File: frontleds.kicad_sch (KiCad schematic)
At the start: 2 parts

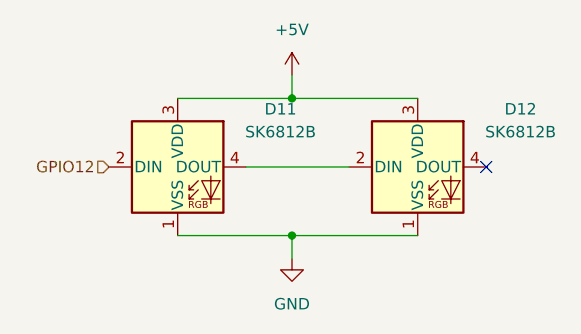
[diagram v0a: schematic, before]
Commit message: finished adding front leds
probably works idk
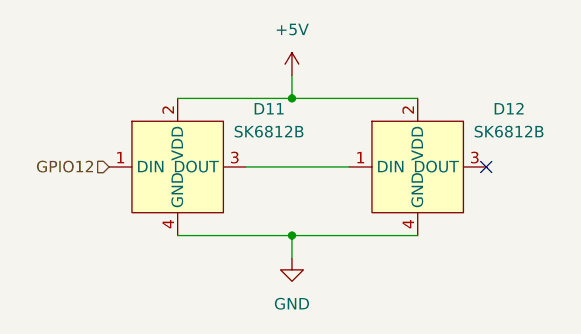
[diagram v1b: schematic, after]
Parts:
- D11, D12: footprint LED_SMD:LED_SK6812_PLCC4_5.0x5.0mm_P3.2mm -> LED_SMD:LED_SK6812B_SIDE_4.0mmx1.5mm
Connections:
- net +5V: now also D11.2 (VDD), D12.2 (VDD); no longer D11.3 (VDD), D12.3 (VDD)
- net GND: now also D11.4 (GND), D12.4 (GND); no longer D11.1 (VSS), D12.1 (VSS)
- net GPIO12: now also D11.1 (DIN); no longer D11.2 (DIN)
- new net: D11.3 (DOUT), D12.1 (DIN)
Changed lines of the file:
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@@
+	)
+	(symbol
+		(lib_id "LED:SK6812B")
+		(at 55.88 29.21 0)
+		(unit 1)
+		(exclude_from_sim no)
+		(in_bom yes)
+		(on_board yes)
+		(dnp no)
+		(fields_autoplaced yes)
+		(property "Reference" "D12"
+			(at 66.04 22.7898 0)
+			(effects
+				(font
+					(size 1.27 1.27)
+				)
+			)
+		)
+		(property "Value" "SK6812B"
+			(at 66.04 25.3298 0)
+			(effects
+				(font
+					(size 1.27 1.27)
+				)
+			)
+		)
+		(property "Footprint" "LED_SMD:LED_SK6812B_SIDE_4.0mmx1.5mm"
+			(at 55.88 29.21 0)
+			(effects
+				(font
+					(size 1.27 1.27)
+				)
+				(hide yes)
+			)
+		)
+		(property "Datasheet" "https://core-electronics.com.au/attachments/localcontent/4691_SK68XX_SIDE_REV_55747b5a68c.pdf"
+			(at 55.88 10.16 0)
+			(effects
+				(font
+					(size 1.27 1.27)
+				)
+				(hide yes)
+			)
+		)
+		(property "Description" "RGB LED with integrated controller"
+			(at 55.88 7.62 0)
+			(effects
+				(font
+					(size 1.27 1.27)
+				)
+				(hide yes)
+			)
+		)
+		(pin "3"
+		)
+		(pin "1"
+		)
+		(pin "4"
+		)
+		(pin "2"
+		)
+		(instances
+			(project "robot_pcb"
+				(path "/2f56b371-1597-47e1-a48d-b7f69d342f77/f9fd353d-136c-4b1d-af31-404dc5242855"
+					(reference "D12")
+					(unit 1)
+				)
+			)
+		)
 	)
 	(symbol
@@
 	)
 	(symbol
+		(lib_id "power:GND")
+		(at 41.91 39.37 0)
+		(unit 1)
+		(exclude_from_sim no)
+		(in_bom yes)
+		(on_board yes)
+		(dnp no)
+		(fields_autoplaced yes)
+		(property "Reference" "#PWR0121"
+			(at 41.91 45.72 0)
+			(effects
+				(font
+					(size 1.27 1.27)
+				)
+				(hide yes)
+			)
+		)
+		(property "Value" "GND"
+			(at 41.91 44.45 0)
+			(effects
+				(font
+					(size 1.27 1.27)
+				)
+			)
+		)
+		(property "Footprint" ""
+			(at 41.91 39.37 0)
+			(effects
+				(font
+					(size 1.27 1.27)
+				)
+				(hide yes)
+			)
+		)
+		(property "Datasheet" ""
+			(at 41.91 39.37 0)
+			(effects
+				(font
+					(size 1.27 1.27)
+				)
+				(hide yes)
+			)
+		)
+		(property "Description" "Power symbol creates a global label with name \"GND\" , ground"
+			(at 41.91 39.37 0)
+			(effects
+				(font
+					(size 1.27 1.27)
+				)
+				(hide yes)
+			)
+		)
+		(pin "1"
+		)
+		(instances
+			(project ""
+				(path "/2f56b371-1597-47e1-a48d-b7f69d342f77/f9fd353d-136c-4b1d-af31-404dc5242855"
+					(reference "#PWR0121")
+					(unit 1)
+				)
+			)
+		)
+	)
+	(symbol
 		(lib_id "LED:SK6812B")
 		(at 29.21 29.21 0)
@@
 		(fields_autoplaced yes)
 		(property "Reference" "D11"
-			(at 40.64 22.7898 0)
+			(at 39.37 22.7898 0)
 			(effects
 				(font
@@
 		)
 		(property "Value" "SK6812B"
-			(at 40.64 25.3298 0)
-			(effects
-				(font
-					(size 1.27 1.27)
-				)
-			)
-		)
-		(property "Footprint" "LED_SMD:LED_SK6812_PLCC4_5.0x5.0mm_P3.2mm"
-			(at 30.48 36.83 0)
-			(effects
-				(font
-					(size 1.27 1.27)
-				)
-				(justify left top)
+			(at 39.37 25.3298 0)
+			(effects
+				(font
+					(size 1.27 1.27)
+				)
+			)
+		)
+		(property "Footprint" "LED_SMD:LED_SK6812B_SIDE_4.0mmx1.5mm"
+			(at 29.21 29.21 0)
+			(effects
+				(font
+					(size 1.27 1.27)
+				)
 				(hide yes)
 			)
 		)
 		(property "Datasheet" "https://core-electronics.com.au/attachments/localcontent/4691_SK68XX_SIDE_REV_55747b5a68c.pdf"
-			(at 31.75 38.735 0)
-			(effects
-				(font
-					(size 1.27 1.27)
-				)
-				(justify left top)
-				(hide yes)
-			)
-		)
-		(property "Description" "Side-light RGB LED with integrated controller"
-			(at 29.21 29.21 0)
-			(effects
-				(font
-					(size 1.27 1.27)
-				)
-				(hide yes)
-			)
+			(at 29.21 10.16 0)
+			(effects
+				(font
+					(size 1.27 1.27)
+				)
+				(hide yes)
+			)
+		)
+		(property "Description" "RGB LED with integrated controller"
+			(at 29.21 7.62 0)
+			(effects
+				(font
+					(size 1.27 1.27)
+				)
+				(hide yes)
+			)
+		)
+		(pin "3"
+		)
+		(pin "1"
+		)
+		(pin "4"
 		)
 		(pin "2"
 		)
-		(pin "1"
-		)
-		(pin "4"
-		)
-		(pin "3"
-		)
 		(instances
 			(project ""
@@
 					(unit 1)
 				)
-			)
-		)
-	)
-	(symbol
-		(lib_id "power:GND")
-		(at 41.91 39.37 0)
-		(unit 1)
-		(exclude_from_sim no)
-		(in_bom yes)
-		(on_board yes)
-		(dnp no)
-		(fields_autoplaced yes)
-		(property "Reference" "#PWR0121"
-			(at 41.91 45.72 0)
-			(effects
-				(font
-					(size 1.27 1.27)
-				)
-				(hide yes)
-			)
-		)
-		(property "Value" "GND"
-			(at 41.91 44.45 0)
-			(effects
-				(font
-					(size 1.27 1.27)
-				)
-			)
-		)
-		(property "Footprint" ""
-			(at 41.91 39.37 0)
-			(effects
-				(font
-					(size 1.27 1.27)
-				)
-				(hide yes)
-			)
-		)
-		(property "Datasheet" ""
-			(at 41.91 39.37 0)
-			(effects
-				(font
-					(size 1.27 1.27)
-				)
-				(hide yes)
-			)
-		)
-		(property "Description" "Power symbol creates a global label with name \"GND\" , ground"
-			(at 41.91 39.37 0)
-			(effects
-				(font
-					(size 1.27 1.27)
-				)
-				(hide yes)
-			)
-		)
-		(pin "1"
-		)
-		(instances
-			(project ""
-				(path "/2f56b371-1597-47e1-a48d-b7f69d342f77/f9fd353d-136c-4b1d-af31-404dc5242855"
-					(reference "#PWR0121")
-					(unit 1)
-				)
-			)
-		)
-	)
-	(symbol
-		(lib_id "LED:SK6812B")
-		(at 55.88 29.21 0)
-		(unit 1)
-		(exclude_from_sim no)
-		(in_bom yes)
-		(on_board yes)
-		(dnp no)
-		(fields_autoplaced yes)
-		(property "Reference" "D12"
-			(at 67.31 22.7898 0)
-			(effects
-				(font
-					(size 1.27 1.27)
-				)
-			)
-		)
-		(property "Value" "SK6812B"
-			(at 67.31 25.3298 0)
-			(effects
-				(font
-					(size 1.27 1.27)
-				)
-			)
-		)
-		(property "Footprint" "LED_SMD:LED_SK6812_PLCC4_5.0x5.0mm_P3.2mm"
-			(at 57.15 36.83 0)
-			(effects
-				(font
-					(size 1.27 1.27)
-				)
-				(justify left top)
-				(hide yes)
-			)
-		)
-		(property "Datasheet" "https://core-electronics.com.au/attachments/localcontent/4691_SK68XX_SIDE_REV_55747b5a68c.pdf"
-			(at 58.42 38.735 0)
-			(effects
-				(font
-					(size 1.27 1.27)
-				)
-				(justify left top)
-				(hide yes)
-			)
-		)
-		(property "Description" "Side-light RGB LED with integrated controller"
-			(at 55.88 29.21 0)
-			(effects
-				(font
-					(size 1.27 1.27)
-				)
-				(hide yes)
-			)
-		)
-		(pin "2"
-		)
-		(pin "1"
-		)
-		(pin "4"
-		)
-		(pin "3"
-		)
-		(instances
-			(project "robot_pcb"
-				(path "/2f56b371-1597-47e1-a48d-b7f69d342f77/f9fd353d-136c-4b1d-af31-404dc5242855"
-					(reference "D12")
-					(unit 1)
-				)

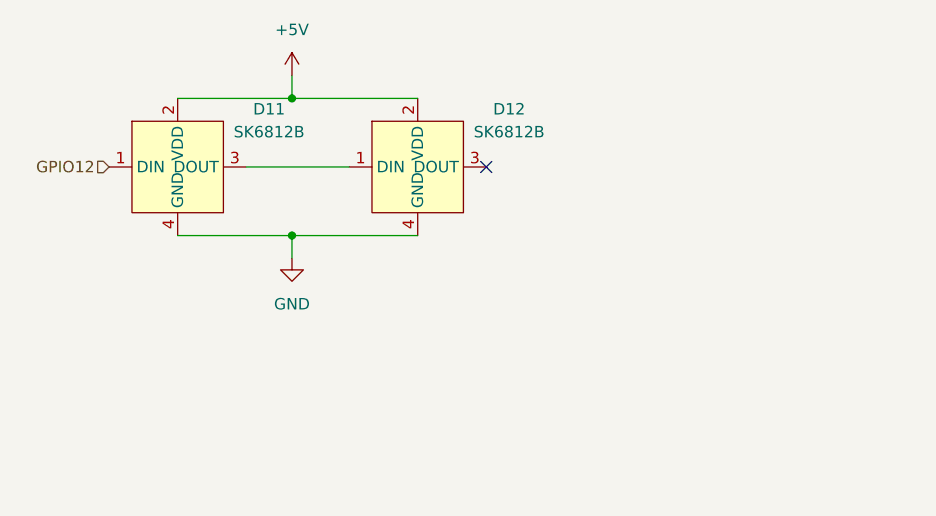
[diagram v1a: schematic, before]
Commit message: send help
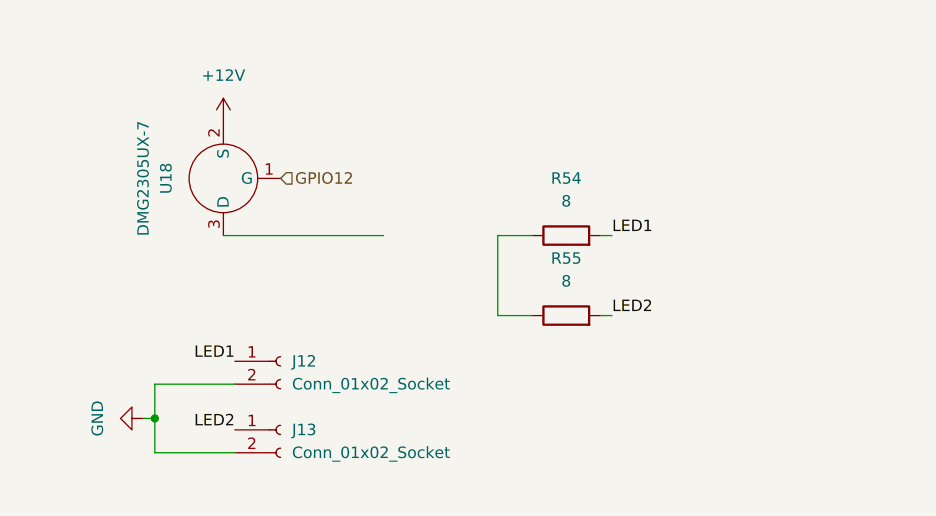
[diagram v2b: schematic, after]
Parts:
- removed D11, D12: SK6812B, LED_SMD:LED_SK6812B_SIDE_4.0mmx1.5mm, symbol LED:SK6812B
- added J12, J13: Conn_01x02_Socket, Connector:JWT_A3963_1x02_P3.96mm_Vertical, symbol Connector:Conn_01x02_Socket
- added R54, R55: 8, Resistor_SMD:R_0402_1005Metric, symbol Device:R
- added U18: DMG2305UX-7, Package_TO_SOT_SMD:TSOT-23, symbol Transistor_FET:DMG2305UX-7
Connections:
- net GND: now also J12.2 (Pin_2), J13.2 (Pin_2)
- net GPIO12: now also U18.1 (G)
- new net: R54.1, R55.1
- new net +12V: U18.2 (S)
- new net LED1: J12.1 (Pin_1), R54.2
- new net LED2: J13.1 (Pin_1), R55.2
- no-connect marks 1 -> 0

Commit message: more stuff with switches n things
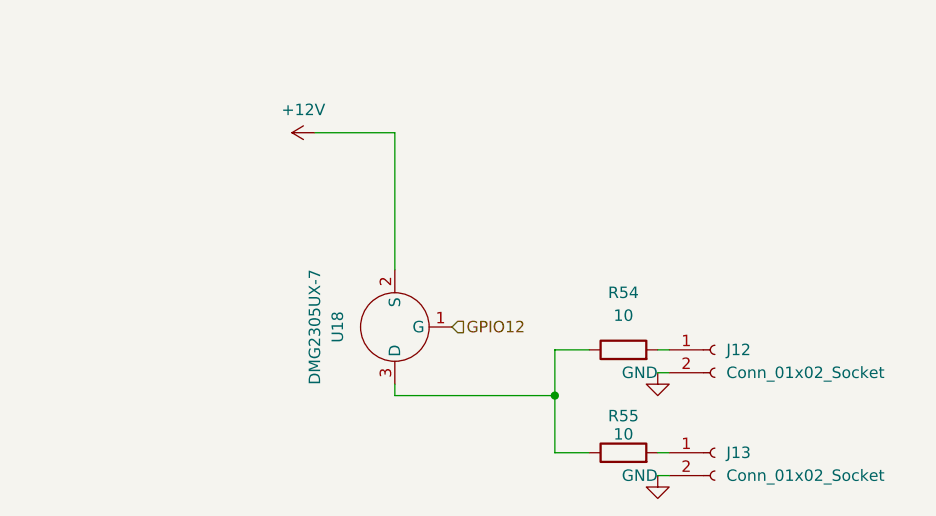
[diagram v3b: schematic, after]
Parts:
- R54, R55: value 8 -> 10
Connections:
- net at R54.1, R55.1: now also U18.3 (D)
- net LED1: no longer names the net of J12.1 (Pin_1), R54.2
- net LED2: no longer names the net of J13.1 (Pin_1), R55.2
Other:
- moved on the sheet: J12, J13, R54, R55, U18
